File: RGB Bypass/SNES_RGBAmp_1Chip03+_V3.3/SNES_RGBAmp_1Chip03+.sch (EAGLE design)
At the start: 32 parts

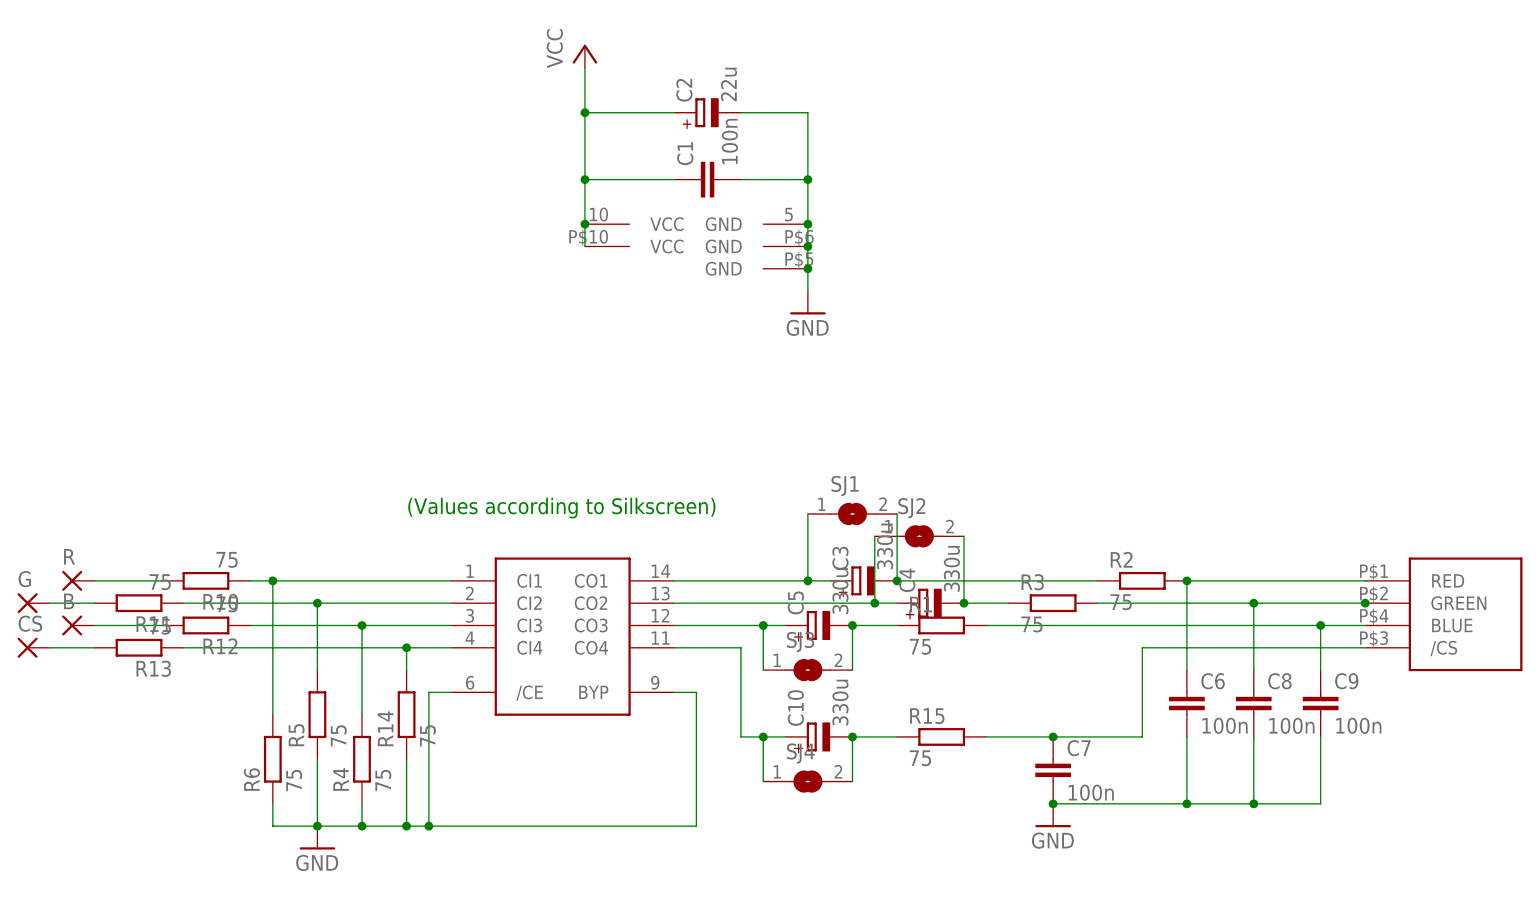
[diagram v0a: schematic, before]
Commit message: Update silkscreen
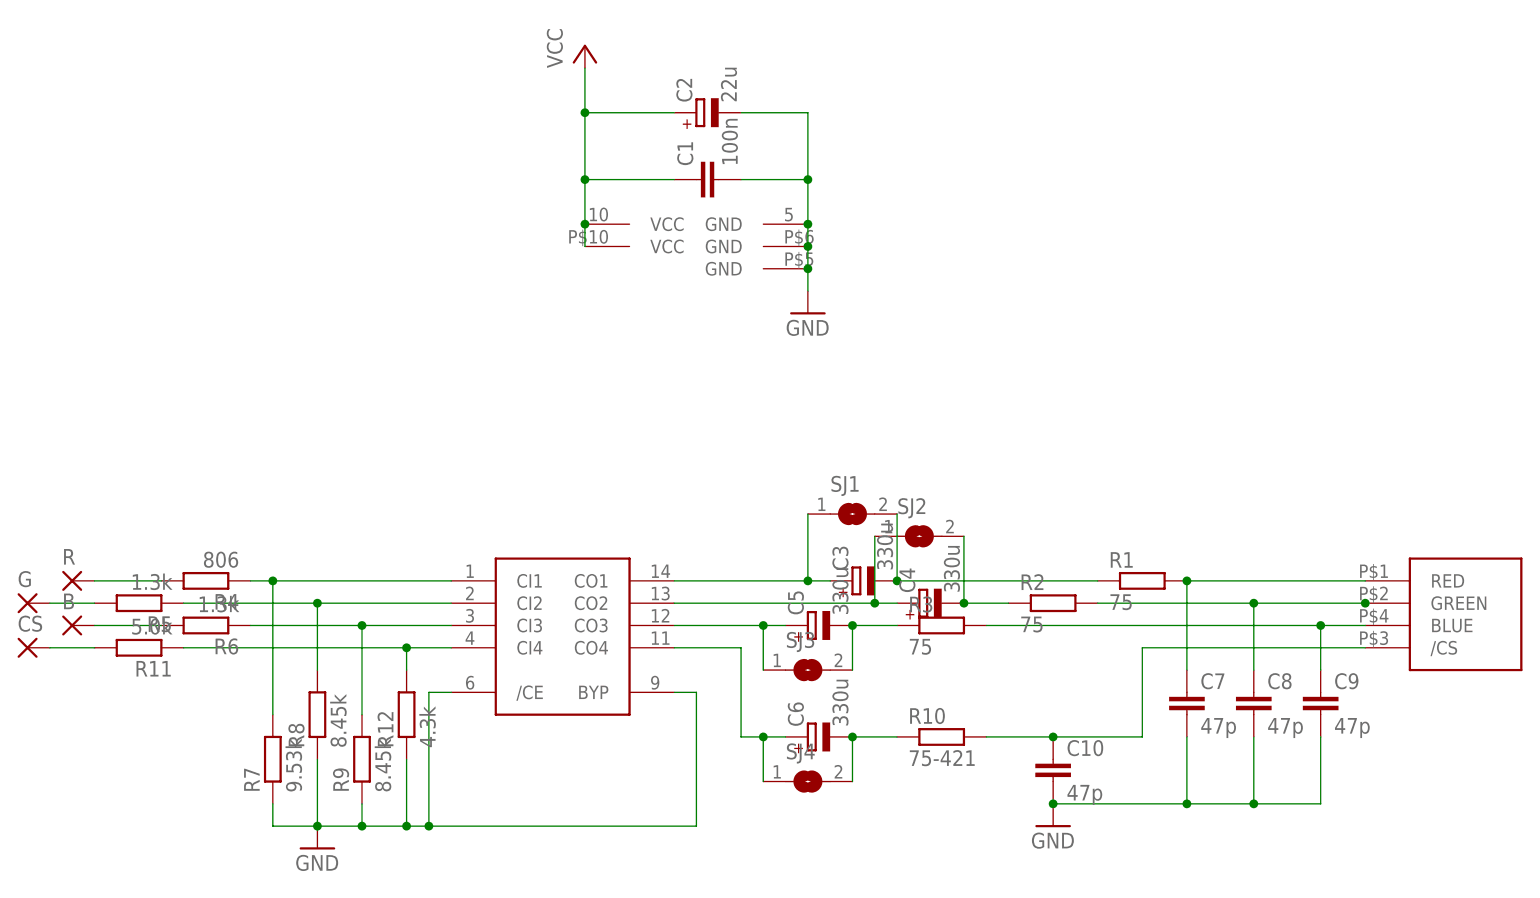
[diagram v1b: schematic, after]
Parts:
- removed R13, R14, R15: 75, snescart:R0805
- added R7: 9.53k, snescart:R0805
- added R8, R9: 8.45k, snescart:R0805
- C10: value 330u -> 47p; device rcl:CPOL-EUSMCD -> snescart:C0805
- C6: value 100n -> 330u; device snescart:C0805 -> rcl:CPOL-EUSMCD
- C7, C8, C9: value 100n -> 47p
- R10: value 75 -> 75-421
- R11: value 75 -> 5.0k
- R12: value 75 -> 4.3k
- R4: value 75 -> 806
- R5, R6: value 75 -> 1.3k
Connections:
- removed net N$3: R12.1, R4.2, U$2G$1.CI3
- new net R9: R6.1, R9.2, U$2G$1.CI3
- net GND: now also C10.2, R12.1, R7.1, R8.1, R9.1; no longer C6.2, R14.1, R4.1, R5.1, R6.1
- net N$1: now also R4.1, R7.2; no longer R10.1, R6.2
- net N$10: now also R11.1, R12.2; no longer R13.1, R14.2
- net N$13: now also R2.1; no longer R3.1
- net N$14: now also R4.2; no longer R10.2
- net N$15: now also R5.2; no longer R11.2
- net N$16: now also R6.2; no longer R12.2
- net N$17: now also R11.2; no longer R13.2
- net N$18: now also C6.+; no longer C10.+
- net N$19: now also C6.-, R10.1; no longer C10.-, R15.1
- net N$2: now also R5.1, R8.2; no longer R11.1, R5.2
- net N$20: now also C10.1, R10.2; no longer C7.1, R15.2
- net N$4: now also R1.1; no longer R2.1
- net N$5: now also C7.1, R1.2; no longer C6.1, R2.2
- net N$6: now also R2.2; no longer R3.2
- net N$8: now also R3.1; no longer R1.1
- net N$9: now also R3.2; no longer R1.2
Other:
- note removed: "(Values according to Silkscreen)"
- moved on the sheet: C7, R1, R10, R11, R12, R2, R3, R4, R5, R6
